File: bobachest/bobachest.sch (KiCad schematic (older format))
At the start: 37 parts, among them Q1 PN2222A, Q2 PN2222A, Q3 PN2222A, Q4 PN2222A, Q5 PN2222A, U1 arduino_mini

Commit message: update
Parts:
- removed R11, R12, R13, R14, R15: R, symbol R
- added RV1: POT, Potentiometers:Potentiometer_Bourns_3339H_Angular_ScrewUp, symbol POT
- AFF1, AFF2, AFF3, AFF4, AFF5: footprint (none) -> 7Segment:7Segment9.9; symbol 7SEGMENTS -> 7SEGMENTS-RESCUE-bobachest
- BAR1, BAR2: footprint (none) -> Display:HDSP-48xx
- Q1, Q2, Q3, Q4, Q5: footprint (none) -> TO_SOT_Packages_THT:TO-92_Inline_Narrow_Oval
- R1, R10, R2, R3, R4, R5, R6, R7, R8, R9: footprint (none) -> Resistors_ThroughHole:Resistor_Horizontal_RM7mm
- R11: renamed from R16; footprint (none) -> Resistors_ThroughHole:Resistor_Horizontal_RM7mm
- R12: renamed from R17; footprint (none) -> Resistors_ThroughHole:Resistor_Horizontal_RM7mm
- R13: renamed from R18; footprint (none) -> Resistors_ThroughHole:Resistor_Horizontal_RM7mm
- R14: renamed from R19; footprint (none) -> Resistors_ThroughHole:Resistor_Horizontal_RM7mm
- R15: renamed from R20; footprint (none) -> Resistors_ThroughHole:Resistor_Horizontal_RM7mm
- R16: renamed from R21; footprint (none) -> Resistors_ThroughHole:Resistor_Horizontal_RM7mm
- R17: renamed from R22; footprint (none) -> Resistors_ThroughHole:Resistor_Horizontal_RM7mm
- R18: renamed from R23; footprint (none) -> Resistors_ThroughHole:Resistor_Horizontal_RM7mm
- RV2: renamed from RV1; footprint (none) -> Potentiometers:Potentiometer_Bourns_3339H_Angular_ScrewUp
- U1: footprint DIL20 -> arduino:arduino_mini
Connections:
- net GND: now also RV1.3; no longer Q1.1 (E), Q2.1 (E), Q3.1 (E), Q4.1 (E), Q5.1 (E)
- net S1: now also U1.28 ((SS)#D10)
- net S2: now also U1.29 ((MOSI)#D11)
- net S3: now also U1.30 ((MISO)D12)
- net S4: now also U1.4 (A0)
- net S5: now also U1.5 (A1)
- net Sa: now also AFF1.10 (a), AFF2.10 (a), AFF3.10 (a), AFF4.10 (a), AFF5.10 (a); no longer AFF1.7 (a), AFF2.7 (a), AFF3.7 (a), AFF4.7 (a), AFF5.7 (a)
- net Sb: now also AFF1.9 (b), AFF2.9 (b), AFF3.9 (b), AFF4.9 (b), AFF5.9 (b); no longer AFF1.6 (b), AFF2.6 (b), AFF3.6 (b), AFF4.6 (b), AFF5.6 (b)
- net Sc: now also AFF1.7 (c), AFF2.7 (c), AFF3.7 (c), AFF4.7 (c), AFF5.7 (c); no longer AFF1.4 (c), AFF2.4 (c), AFF3.4 (c), AFF4.4 (c), AFF5.4 (c)
- net Sd: now also AFF1.5 (d), AFF2.5 (d), AFF3.5 (d), AFF4.5 (d), AFF5.5 (d); no longer AFF1.2 (d), AFF2.2 (d), AFF3.2 (d), AFF4.2 (d), AFF5.2 (d)
- net Se: now also AFF1.4 (e), AFF2.4 (e), AFF3.4 (e), AFF4.4 (e), AFF5.4 (e); no longer AFF1.1 (e), AFF2.1 (e), AFF3.1 (e), AFF4.1 (e), AFF5.1 (e)
- net Sf: now also AFF1.2 (f), AFF2.2 (f), AFF3.2 (f), AFF4.2 (f), AFF5.2 (f); no longer AFF1.9 (f), AFF2.9 (f), AFF3.9 (f), AFF4.9 (f), AFF5.9 (f)
- net Sg: now also AFF1.1 (g), AFF2.1 (g), AFF3.1 (g), AFF4.1 (g), AFF5.1 (g); no longer AFF1.10 (g), AFF2.10 (g), AFF3.10 (g), AFF4.10 (g), AFF5.10 (g)
- net Sp: now also AFF1.6 (DP), AFF2.6 (DP), AFF3.6 (DP), AFF4.6 (DP), AFF5.6 (DP); no longer AFF1.5 (DP), AFF2.5 (DP), AFF3.5 (DP), AFF4.5 (DP), AFF5.5 (DP)
- new net: Q1.1 (E), Q2.1 (E), Q3.1 (E), Q4.1 (E), Q5.1 (E), RV1.2
- no-connect marks 10 -> 11

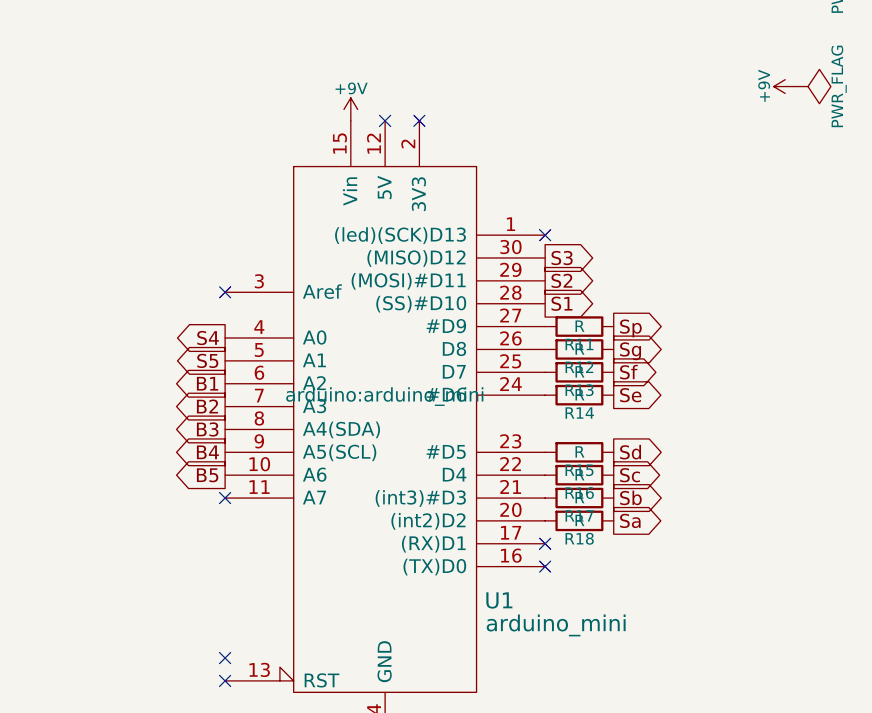
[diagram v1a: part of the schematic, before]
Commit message: Bobachest update
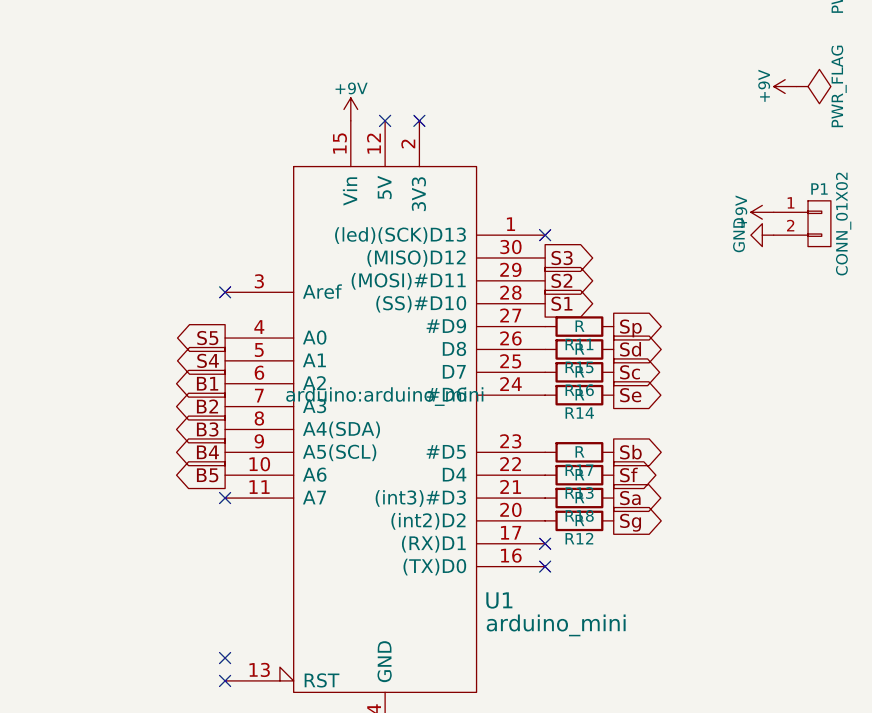
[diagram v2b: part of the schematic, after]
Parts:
- added P1: CONN_01X02, Pin_Headers:Pin_Header_Straight_1x02, symbol CONN_01X02
- BAR1, BAR2: footprint Display:HDSP-48xx -> BarSegm:HDSP-48xx
- R1, R10, R11, R12, R13, R14, R15, R16, R17, R18, R2, R3, R4, R5, R6, R7, R8, R9: footprint Resistors_ThroughHole:Resistor_Horizontal_RM7mm -> Resistor7mm:Resistor_Horizontal_RM7mm
- RV1, RV2: footprint Potentiometers:Potentiometer_Bourns_3339H_Angular_ScrewUp -> TRIMPOT:Potentiometer_Trimmer-Suntan-TSR-3386P
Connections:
- net +9V: now also P1.1 (P1)
- net GND: now also P1.2 (P2)
- net S4: now also U1.5 (A1); no longer U1.4 (A0)
- net S5: now also U1.4 (A0); no longer U1.5 (A1)
- net at R18.2: now also U1.21 ((int3)#D3); no longer U1.20 ((int2)D2)
- net at R17.2: now also U1.23 (#D5); no longer U1.21 ((int3)#D3)
- net at R16.2: now also U1.25 (D7); no longer U1.22 (D4)
- net at R15.2: now also U1.26 (D8); no longer U1.23 (#D5)
- net at R13.2: now also U1.22 (D4); no longer U1.25 (D7)
- net at R12.2: now also U1.20 ((int2)D2); no longer U1.26 (D8)
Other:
- moved on the sheet: R12, R13, R15, R16, R17, R18
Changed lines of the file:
@@
 F 0 "R1" V 3080 1600 50  0000 C CNN
 F 1 "R" V 3000 1600 50  0000 C CNN
-F 2 "Resistors_ThroughHole:Resistor_Horizontal_RM7mm" V 2930 1600 50  0001 C CNN
+F 2 "Resistor7mm:Resistor_Horizontal_RM7mm" V 2930 1600 50  0001 C CNN
 F 3 "" H 3000 1600 50  0000 C CNN
 	1    3000 1600
@@
 F 0 "R2" V 3080 2850 50  0000 C CNN
 F 1 "R" V 3000 2850 50  0000 C CNN
-F 2 "Resistors_ThroughHole:Resistor_Horizontal_RM7mm" V 2930 2850 50  0001 C CNN
+F 2 "Resistor7mm:Resistor_Horizontal_RM7mm" V 2930 2850 50  0001 C CNN
 F 3 "" H 3000 2850 50  0000 C CNN
 	1    3000 2850
@@
 F 0 "R3" V 3080 4100 50  0000 C CNN
 F 1 "R" V 3000 4100 50  0000 C CNN
-F 2 "Resistors_ThroughHole:Resistor_Horizontal_RM7mm" V 2930 4100 50  0001 C CNN
+F 2 "Resistor7mm:Resistor_Horizontal_RM7mm" V 2930 4100 50  0001 C CNN
 F 3 "" H 3000 4100 50  0000 C CNN
 	1    3000 4100
@@
 F 0 "R4" V 3080 5350 50  0000 C CNN
 F 1 "R" V 3000 5350 50  0000 C CNN
-F 2 "Resistors_ThroughHole:Resistor_Horizontal_RM7mm" V 2930 5350 50  0001 C CNN
+F 2 "Resistor7mm:Resistor_Horizontal_RM7mm" V 2930 5350 50  0001 C CNN
 F 3 "" H 3000 5350 50  0000 C CNN
 	1    3000 5350
@@
 F 0 "R5" V 3080 6600 50  0000 C CNN
 F 1 "R" V 3000 6600 50  0000 C CNN
-F 2 "Resistors_ThroughHole:Resistor_Horizontal_RM7mm" V 2930 6600 50  0001 C CNN
+F 2 "Resistor7mm:Resistor_Horizontal_RM7mm" V 2930 6600 50  0001 C CNN
 F 3 "" H 3000 6600 50  0000 C CNN
 	1    3000 6600
@@
 F 0 "BAR1" H 5400 4000 50  0000 C CNN
 F 1 "DOT-BAR2" H 5500 3850 50  0000 C CNN
-F 2 "Display:HDSP-48xx" H 5500 2550 50  0001 C CNN
+F 2 "BarSegm:HDSP-48xx" H 5500 2550 50  0001 C CNN
 F 3 "" H 5500 2550 50  0000 C CNN
 	1    5500 2550
@@
 F 0 "BAR2" H 5400 6800 50  0000 C CNN
 F 1 "DOT-BAR2" H 5500 6650 50  0000 C CNN
-F 2 "Display:HDSP-48xx" H 5500 5350 50  0001 C CNN
+F 2 "BarSegm:HDSP-48xx" H 5500 5350 50  0001 C CNN
 F 3 "" H 5500 5350 50  0000 C CNN
 	1    5500 5350
@@
 F 0 "R6" V 4880 1450 50  0000 C CNN
 F 1 "R" V 4800 1450 50  0000 C CNN
-F 2 "Resistors_ThroughHole:Resistor_Horizontal_RM7mm" V 4730 1450 50  0001 C CNN
+F 2 "Resistor7mm:Resistor_Horizontal_RM7mm" V 4730 1450 50  0001 C CNN
 F 3 "" H 4800 1450 50  0000 C CNN
 	1    4800 1450
@@
 F 0 "R7" V 4880 2450 50  0000 C CNN
 F 1 "R" V 4800 2450 50  0000 C CNN
-F 2 "Resistors_ThroughHole:Resistor_Horizontal_RM7mm" V 4730 2450 50  0001 C CNN
+F 2 "Resistor7mm:Resistor_Horizontal_RM7mm" V 4730 2450 50  0001 C CNN
 F 3 "" H 4800 2450 50  0000 C CNN
 	1    4800 2450
@@
 F 0 "R8" V 4880 3450 50  0000 C CNN
 F 1 "R" V 4800 3450 50  0000 C CNN
-F 2 "Resistors_ThroughHole:Resistor_Horizontal_RM7mm" V 4730 3450 50  0001 C CNN
+F 2 "Resistor7mm:Resistor_Horizontal_RM7mm" V 4730 3450 50  0001 C CNN
 F 3 "" H 4800 3450 50  0000 C CNN
 	1    4800 3450
@@
 F 0 "R9" V 4880 4750 50  0000 C CNN
 F 1 "R" V 4800 4750 50  0000 C CNN
-F 2 "Resistors_ThroughHole:Resistor_Horizontal_RM7mm" V 4730 4750 50  0001 C CNN
+F 2 "Resistor7mm:Resistor_Horizontal_RM7mm" V 4730 4750 50  0001 C CNN
 F 3 "" H 4800 4750 50  0000 C CNN
 	1    4800 4750
@@
 F 0 "R10" V 4880 5750 50  0000 C CNN
 F 1 "R" V 4800 5750 50  0000 C CNN
-F 2 "Resistors_ThroughHole:Resistor_Horizontal_RM7mm" V 4730 5750 50  0001 C CNN
+F 2 "Resistor7mm:Resistor_Horizontal_RM7mm" V 4730 5750 50  0001 C CNN
 F 3 "" H 4800 5750 50  0000 C CNN
 	1    4800 5750
@@
 L R R18
 U 1 1 5840A238
-P 9300 4150
-F 0 "R18" V 9380 4150 50  0000 C CNN
-F 1 "R" V 9300 4150 50  0000 C CNN
-F 2 "Resistors_ThroughHole:Resistor_Horizontal_RM7mm" V 9230 4150 50  0001 C CNN
-F 3 "" H 9300 4150 50  0000 C CNN
-	1    9300 4150
+P 9300 4050
+F 0 "R18" V 9380 4050 50  0000 C CNN
+F 1 "R" V 9300 4050 50  0000 C CNN
+F 2 "Resistor7mm:Resistor_Horizontal_RM7mm" V 9230 4050 50  0001 C CNN
+F 3 "" H 9300 4050 50  0000 C CNN
+	1    9300 4050
 	0    1    1    0
 $EndComp
@@
 L R R17
 U 1 1 5840A3D8
-P 9300 4050
-F 0 "R17" V 9380 4050 50  0000 C CNN
-F 1 "R" V 9300 4050 50  0000 C CNN
-F 2 "Resistors_ThroughHole:Resistor_Horizontal_RM7mm" V 9230 4050 50  0001 C CNN
-F 3 "" H 9300 4050 50  0000 C CNN
-	1    9300 4050
+P 9300 3850
+F 0 "R17" V 9380 3850 50  0000 C CNN
+F 1 "R" V 9300 3850 50  0000 C CNN
+F 2 "Resistor7mm:Resistor_Horizontal_RM7mm" V 9230 3850 50  0001 C CNN
+F 3 "" H 9300 3850 50  0000 C CNN
+	1    9300 3850
 	0    1    1    0
 $EndComp
@@
 L R R16
 U 1 1 5840A437
-P 9300 3950
-F 0 "R16" V 9380 3950 50  0000 C CNN
-F 1 "R" V 9300 3950 50  0000 C CNN
-F 2 "Resistors_ThroughHole:Resistor_Horizontal_RM7mm" V 9230 3950 50  0001 C CNN
-F 3 "" H 9300 3950 50  0000 C CNN
-	1    9300 3950
+P 9300 3500
+F 0 "R16" V 9380 3500 50  0000 C CNN
+F 1 "R" V 9300 3500 50  0000 C CNN
+F 2 "Resistor7mm:Resistor_Horizontal_RM7mm" V 9230 3500 50  0001 C CNN
+F 3 "" H 9300 3500 50  0000 C CNN
+	1    9300 3500
 	0    1    1    0
 $EndComp
@@
 L R R15
 U 1 1 5840A495
-P 9300 3850
-F 0 "R15" V 9380 3850 50  0000 C CNN
-F 1 "R" V 9300 3850 50  0000 C CNN
-F 2 "Resistors_ThroughHole:Resistor_Horizontal_RM7mm" V 9230 3850 50  0001 C CNN
-F 3 "" H 9300 3850 50  0000 C CNN
-	1    9300 3850
+P 9300 3400
+F 0 "R15" V 9380 3400 50  0000 C CNN
+F 1 "R" V 9300 3400 50  0000 C CNN
+F 2 "Resistor7mm:Resistor_Horizontal_RM7mm" V 9230 3400 50  0001 C CNN
+F 3 "" H 9300 3400 50  0000 C CNN
+	1    9300 3400
 	0    1    1    0
 $EndComp
@@
 F 0 "R14" V 9380 3600 50  0000 C CNN
 F 1 "R" V 9300 3600 50  0000 C CNN
-F 2 "Resistors_ThroughHole:Resistor_Horizontal_RM7mm" V 9230 3600 50  0001 C CNN
+F 2 "Resistor7mm:Resistor_Horizontal_RM7mm" V 9230 3600 50  0001 C CNN
 F 3 "" H 9300 3600 50  0000 C CNN
 	1    9300 3600
@@
 L R R13
 U 1 1 5840AB2D
-P 9300 3500
-F 0 "R13" V 9380 3500 50  0000 C CNN
-F 1 "R" V 9300 3500 50  0000 C CNN
-F 2 "Resistors_ThroughHole:Resistor_Horizontal_RM7mm" V 9230 3500 50  0001 C CNN
-F 3 "" H 9300 3500 50  0000 C CNN
-	1    9300 3500
+P 9300 3950
+F 0 "R13" V 9380 3950 50  0000 C CNN
+F 1 "R" V 9300 3950 50  0000 C CNN
+F 2 "Resistor7mm:Resistor_Horizontal_RM7mm" V 9230 3950 50  0001 C CNN
+F 3 "" H 9300 3950 50  0000 C CNN
+	1    9300 3950
 	0    1    1    0
 $EndComp
@@
 F 0 "R11" V 9380 3300 50  0000 C CNN
 F 1 "R" V 9300 3300 50  0000 C CNN
-F 2 "Resistors_ThroughHole:Resistor_Horizontal_RM7mm" V 9230 3300 50  0001 C CNN
+F 2 "Resistor7mm:Resistor_Horizontal_RM7mm" V 9230 3300 50  0001 C CNN
 F 3 "" H 9300 3300 50  0000 C CNN
 	1    9300 3300
 	0    1    1    0
 $EndComp
-Text GLabel 9450 4150 2    60   Output ~ 0
+Text GLabel 9450 4050 2    60   Output ~ 0
 Sa
-Text GLabel 9450 4050 2    60   Output ~ 0
+Text GLabel 9450 3850 2    60   Output ~ 0
 Sb
-Text GLabel 9450 3950 2    60   Output ~ 0
+Text GLabel 9450 3500 2    60   Output ~ 0
 Sc
-Text GLabel 9450 3850 2    60   Output ~ 0
+Text GLabel 9450 3400 2    60   Output ~ 0
 Sd
 Text GLabel 9450 3600 2    60   Output ~ 0
 Se
-Text GLabel 9450 3500 2    60   Output ~ 0
+Text GLabel 9450 3950 2    60   Output ~ 0
 Sf
 Text GLabel 9450 3300 2    60   Output ~ 0
@@
 S3
 Text GLabel 7750 3350 0    60   Output ~ 0
+S5
+Text GLabel 7750 3450 0    60   Output ~ 0
 S4
-Text GLabel 7750 3450 0    60   Output ~ 0
-S5
 Text GLabel 7750 3550 0    60   Output ~ 0
 B1
@@
 L R R12
 U 1 1 58426843
-P 9300 3400
-F 0 "R12" V 9380 3400 50  0000 C CNN
-F 1 "R" V 9300 3400 50  0000 C CNN
-F 2 "Resistors_ThroughHole:Resistor_Horizontal_RM7mm" V 9230 3400 50  0001 C CNN
-F 3 "" H 9300 3400 50  0000 C CNN
-	1    9300 3400
-	0    1    1    0
-$EndComp
-Text GLabel 9450 3400 2    60   Output ~ 0
+P 9300 4150
+F 0 "R12" V 9380 4150 50  0000 C CNN
+F 1 "R" V 9300 4150 50  0000 C CNN
+F 2 "Resistor7mm:Resistor_Horizontal_RM7mm" V 9230 4150 50  0001 C CNN
+F 3 "" H 9300 4150 50  0000 C CNN
+	1    9300 4150
+	0    1    1    0
+$EndComp
+Text GLabel 9450 4150 2    60   Output ~ 0
 Sg
 NoConn ~ 9150 4350
@@
 F 0 "RV2" H 6200 4120 50  0000 C CNN
 F 1 "POT" H 6200 4200 50  0000 C CNN
-F 2 "Potentiometers:Potentiometer_Bourns_3339H_Angular_ScrewUp" H 6200 4200 50  0001 C CNN
+F 2 "TRIMPOT:Potentiometer_Trimmer-Suntan-TSR-3386P" H 6200 4200 50  0001 C CNN
 F 3 "" H 6200 4200 50  0000 C CNN
 	1    6200 4200
@@
 F 0 "RV1" H 3850 3770 50  0000 C CNN
 F 1 "POT" H 3850 3850 50  0000 C CNN
-F 2 "Potentiometers:Potentiometer_Bourns_3339H_Angular_ScrewUp" H 3850 3850 50  0001 C CNN
+F 2 "TRIMPOT:Potentiometer_Trimmer-Suntan-TSR-3386P" H 3850 3850 50  0001 C CNN
 F 3 "" H 3850 3850 50  0000 C CNN
 	1    3850 3850
@@
 	3300 6150 3200 6150
 Connection ~ 3300 4900
+$Comp
+L CONN_01X02 P1
+U 1 1 5848B695
+P 10350 2850
+F 0 "P1" H 10350 3000 50  0000 C CNN
+F 1 "CONN_01X02" V 10450 2850 50  0000 C CNN
+F 2 "Pin_Headers:Pin_Header_Straight_1x02" H 10350 2850 50  0001 C CNN
+F 3 "" H 10350 2850 50  0000 C CNN
+	1    10350 2850
+	1    0    0    -1
+$EndComp
+$Comp
+L +9V #PWR09
+U 1 1 5848CF48
+P 10150 2800
+F 0 "#PWR09" H 10150 2650 50  0001 C CNN
+F 1 "+9V" H 10150 2940 50  0000 C CNN
+F 2 "" H 10150 2800 50  0000 C CNN
+F 3 "" H 10150 2800 50  0000 C CNN
+	1    10150 2800
+	0    -1   -1   0
+$EndComp
+$Comp
+L GND #PWR010
+U 1 1 5848CFB9
+P 10150 2900
+F 0 "#PWR010" H 10150 2650 50  0001 C CNN
+F 1 "GND" H 10150 2750 50  0000 C CNN
+F 2 "" H 10150 2900 50  0000 C CNN
+F 3 "" H 10150 2900 50  0000 C CNN
+	1    10150 2900
+	0    1    1    0
+$EndComp
 $EndSCHEMATC
